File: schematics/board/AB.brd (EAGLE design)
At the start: 78 x 21 mm, 65 parts

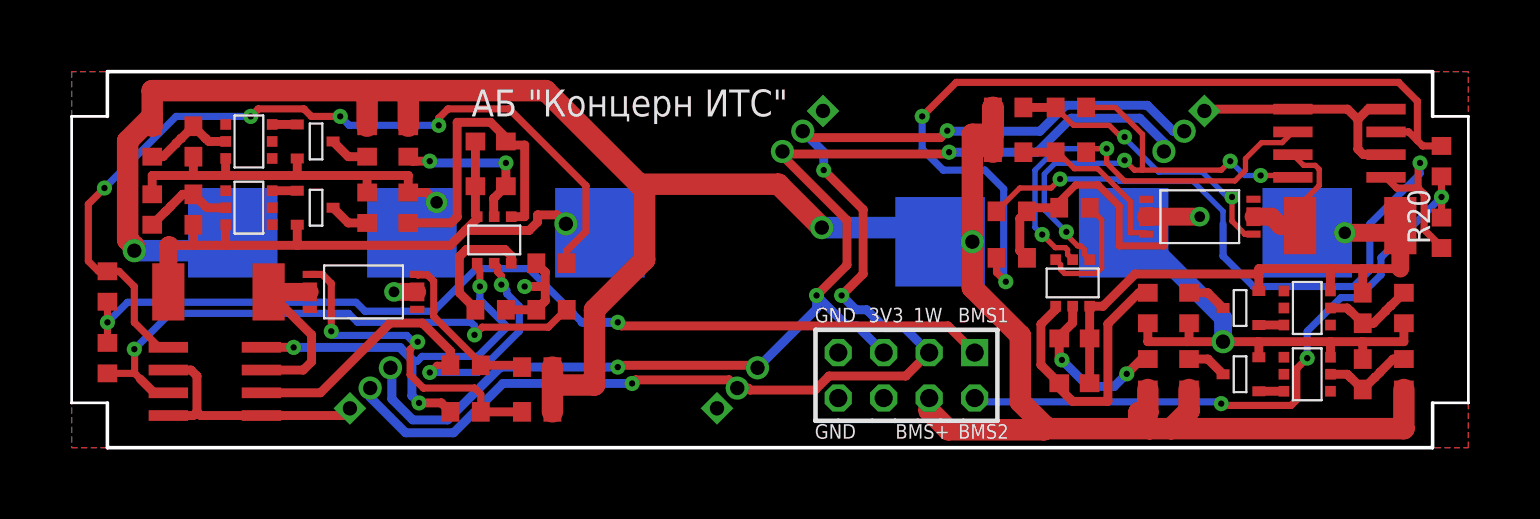
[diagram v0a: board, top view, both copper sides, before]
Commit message: Готова плата RADIO и переделана плата AB
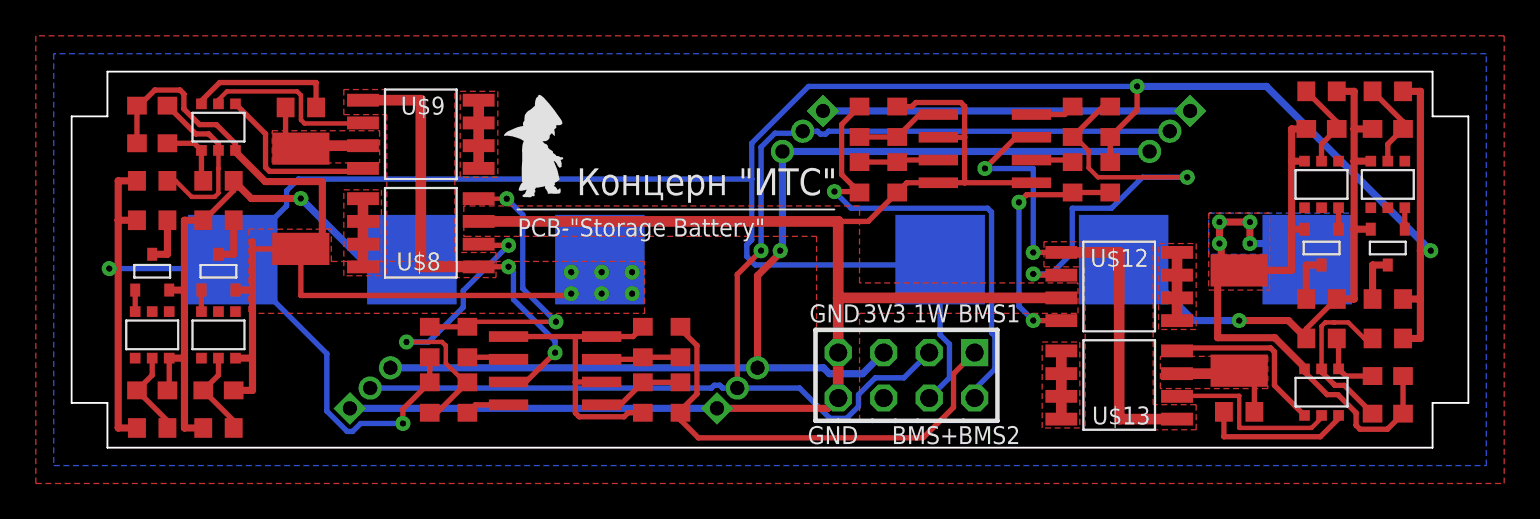
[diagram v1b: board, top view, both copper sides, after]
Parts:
- removed R15, R16: 100R, resistor:R0603
- removed R17, R18: 100k, resistor:R0603
- removed R19, R20: 2k26, resistor:R0603
- removed R98, R99: 200k, resistor:R0603
- removed U$10: MOCD217M, CanCubeSat:SOIC8
- removed U$26: FS8205A-, CanCubeSat:FS8205A-
- added R21, R22: 200k, resistor:R0603
- added R23, R24: 150R, resistor:R0603
- added R25, R26: 10k, resistor:R0603
- added R27, R28: 2k26, resistor:R0603
- added U$11: MOCD217M, CanCubeSat:SOIC8
- added U$12, U$13, U$8, U$9: IRF7905PBF, CanCubeSat:SO8
- DS18B20, DS18B20A, DS18B20B, DS18B20C: value CONNECT1X3 -> DS18B20
- R10, R9: value 100R -> 150R
- R11, R12: value 100k -> 10k
- U$1: value FS8205A- -> PCB-"Storage Battery"; device CanCubeSat:FS8205A- -> CanCubeSat:ITS-LOGO
- moved U$1 38.1 mm to (24.9, 13.3), turned to 0 degrees
- moved R14 32.6 mm to (34.0, 2.80)
- moved R13 32.0 mm to (34.0, 5.90)
- moved C1 19.4 mm to (4.50, 19.1)
- moved U$2 19.0 mm to (27.0, 4.30), turned to 90 degrees
- moved C2 18.9 mm to (4.50, 17.0)
- moved C25 18.0 mm to (73.5, 1.90)
- moved C26 17.5 mm to (73.5, 4.00)
- moved U$3 16.6 mm to (8.20, 17.9), turned to 180 degrees
- moved R6 16.0 mm to (4.50, 1.10), turned to 180 degrees
- moved R54 15.8 mm to (73.5, 19.9), turned to 0 degrees
- moved R1 15.5 mm to (12.8, 19.0), turned to 0 degrees
- moved U$45 15.2 mm to (69.8, 3.10), turned to 0 degrees
- moved R49 14.6 mm to (65.2, 2.00), turned to 180 degrees
- moved R2 14.5 mm to (4.50, 14.9), turned to 180 degrees
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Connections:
- removed net N$10: R16.1, R17.2, U$1.5
- removed net N$14: R15.1, R18.1, U$1.4
- removed net N$19: R19.1, R99.2, U$10.3
- removed net N$3 (its old number): R20.1, R98.2, U$10.1
- new net N$16: U$9.5, U$9.6, U$9.7, U$9.8
- new net N$17: R10.1, U$2.8
- new net N$20: R22.2, R27.1, U$11.3
- new net N$21: U$8.5, U$8.6, U$8.7, U$8.8
- new net N$22: R9.1, U$2.6
- new net N$23: R12.1, R9.2, U$8.4
- new net N$24: R21.2, R28.1, U$11.1
- new net N$26: R24.2, R25.2, U$12.2
- new net N$27: R24.1, U$11.8
- new net N$28: R23.1, U$11.6
- new net N$29: R23.2, R26.1, U$12.4
- new net N$30: U$11.7, U$12.1, U$13.1
- new net N$31: U$13.5, U$13.6, U$13.7, U$13.8
- new net N$32: U$12.5, U$12.6, U$12.7, U$12.8
- net BMS+: now also R25.1, R26.2; no longer R17.1, R18.2
- net BMS2: now also R27.2, R28.2; no longer R19.2, R20.2
- net GND: now also R21.1, R22.1, U$11.2, U$11.4, U$11.5, U$12.3, U$8.3; no longer R1.1, R49.1, R98.1, R99.1, U$1.23, U$10.2, U$10.4, U$10.5, U$26.23
- net N$1: now also U$2.7, U$8.1, U$9.1; no longer R10.1, R11.2, U$26.5
- net N$2: now also R10.2, R11.2, U$8.2; no longer R12.1, R9.1, U$26.4
- net NO_GND1: now also R1.1, U$9.3; no longer U$2.7, U$26.67
- net NO_GND2: now also R49.1, U$13.3; no longer U$1.67, U$10.7
- net OC1: now also U$9.2; no longer R9.2, U$2.6
- net OC2: now also U$13.2; no longer R15.2, U$10.6
- net OD1: now also U$9.4; no longer R10.2, U$2.8
- net OD2: now also U$13.4; no longer R16.2, U$10.8
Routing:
- net GND: track 54.1 -> 129.2 mm, vias 3 -> 0
- net N$19: track 48.6 -> 0.00 mm, vias 2 -> 0
- net N$25: track 48.4 -> 4.92 mm, vias 4 -> 0
- net N$3 (its old number): track 40.4 -> 0.00 mm, vias 2 -> 0
- net BMS1: track 54.3 -> 25.9 mm, vias 2 -> 0
- net N$30: track 0.00 -> 28.1 mm, vias 0 -> 2
- net N$18: track 31.6 -> 4.45 mm, vias 2 -> 0
- net N$26: track 0.00 -> 24.6 mm, vias 0 -> 2
- net B-1: track 36.8 -> 60.5 mm, vias 1 -> 6
- net BMS+: track 145.5 -> 166.9 mm, vias 3 -> 4
- net OD2: track 26.7 -> 9.85 mm, vias 4 -> 0
- net N$23: track 0.00 -> 16.7 mm, vias 0 -> 2
- net N$10: track 16.7 -> 0.00 mm, vias 2 -> 0
- net OC1: track 25.3 -> 10.0 mm, vias 2 -> 0
- net OC2: track 25.1 -> 10.3 mm, vias 2 -> 0
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- added copper zone on layer 1, net B-1
- added copper zone on layer 1, net B-2
- added copper zone on layer 16, net B-2
- added copper zone on layer 16, net BMS+
- added copper zone on layer 1, net GND
- added copper zone on layer 1, net N$1
- added copper zone on layer 1, net N$16
- added copper zone on layer 1, net N$21
- added copper zone on layer 1, net N$30
- added copper zone on layer 1, net N$31
- added copper zone on layer 1, net N$32
- added copper zone on layer 1, net NO_GND1
- added copper zone on layer 1, net NO_GND2
- removed copper zone on layer 1, net BMS+
- removed copper zone on layer 16, net GND
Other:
- board text added: "HY2120"
- board text added: "HY2213"
- board text added: "IRF7905"
- board text added: "SI2302"
- board text removed: "АБ "Концерн ИТС""
